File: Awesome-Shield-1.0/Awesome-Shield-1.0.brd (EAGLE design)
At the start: 51 x 55 mm, 21 parts, among them J1 PORT1, J2 PORT2, J3 PORT3, SW1 SPST_TACT-EVQQ2, SW2 DPDT, U1 LIGHTSENSORTEMT6000, X1 PASSER-07, X2 PASSER-07

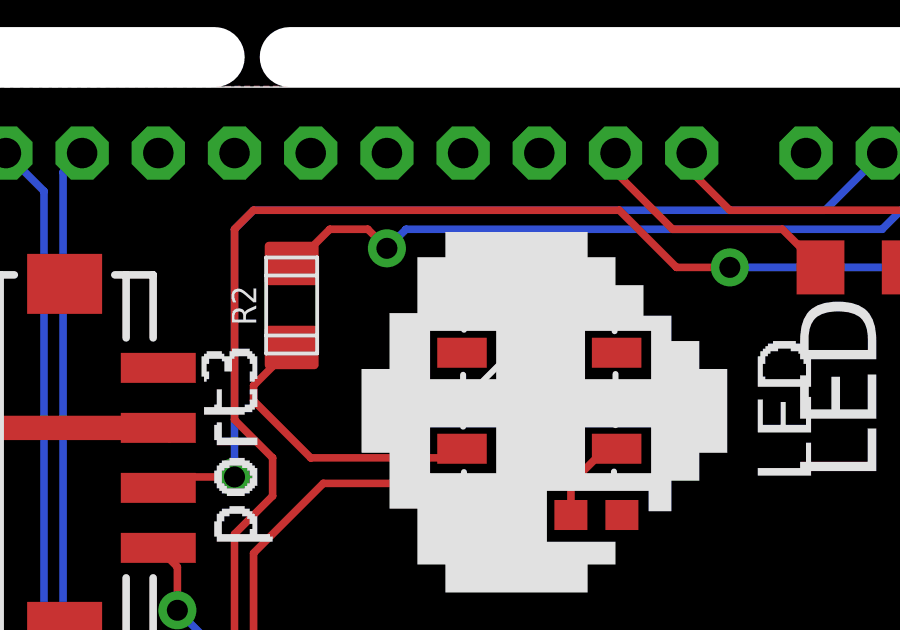
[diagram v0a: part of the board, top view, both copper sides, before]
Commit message: nudged resistor
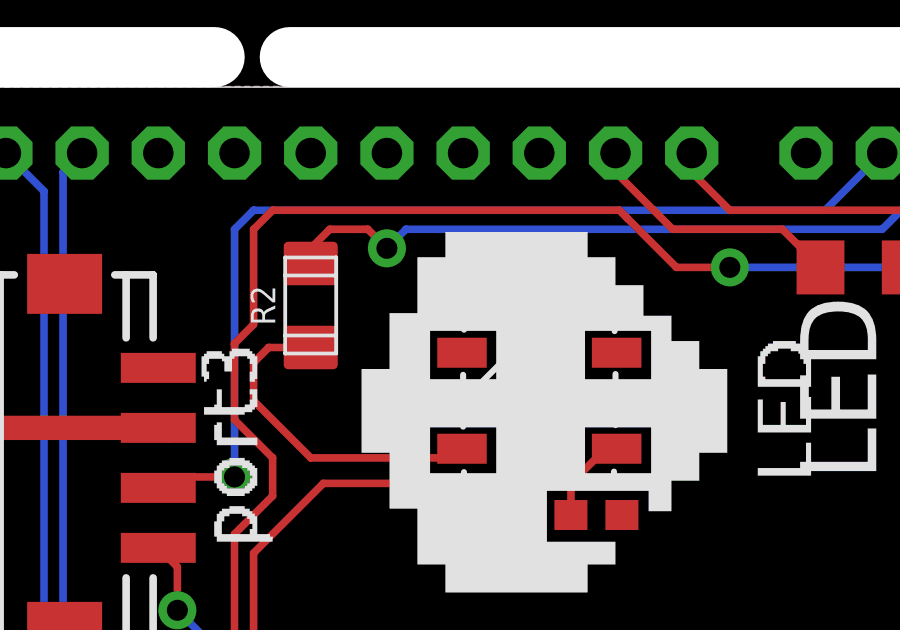
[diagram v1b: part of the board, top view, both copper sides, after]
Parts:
- moved R2 0.63 mm to (12.7, 45.7)
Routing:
- net N$3: track 10.2 -> 11.2 mm
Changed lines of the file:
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@@
 <element name="R1" library="rcl" package="R1206" value="TBD" x="31.115" y="46.99" smashed="yes" rot="R180"/>
 <element name="U$1" library="buzzer-loudity-bzel-t68-0808" package="SMT-68" value="LOUDITY-BZEL-T680808" x="38.735" y="43.18" smashed="yes" rot="R90"/>
-<element name="R2" library="we-rcl" package="C1206" value="330R" x="12.065" y="45.72"/>
+<element name="R2" library="we-rcl" package="C1206" value="330R" x="12.7" y="45.72"/>
 <element name="X1" library="we-symbol" package="PASSER_07MM" value="PASSER-07" x="1.27" y="48.26"/>
 <element name="X2" library="we-symbol" package="PASSER_07MM" value="PASSER-07" x="47.625" y="5.08"/>
@@
 <contactref element="R2" pad="1"/>
 <wire x1="13.335" y1="48.26" x2="12.195" y2="47.12" width="0.254" layer="1"/>
-<wire x1="12.195" y1="47.12" x2="12.065" y2="47.12" width="0.254" layer="1"/>
+<wire x1="12.195" y1="47.12" x2="12.7" y2="47.12" width="0.254" layer="1"/>
 <wire x1="13.335" y1="48.26" x2="14.605" y2="48.26" width="0.254" layer="1"/>
 <wire x1="14.605" y1="48.26" x2="15.24" y2="47.625" width="0.254" layer="1"/>
@@
 <wire x1="11.43" y1="39.37" x2="11.43" y2="40.64" width="0.254" layer="1"/>
 <wire x1="11.43" y1="40.64" x2="10.16" y2="41.91" width="0.254" layer="1"/>
-<wire x1="10.16" y1="41.91" x2="10.16" y2="48.26" width="0.254" layer="1"/>
-<wire x1="10.16" y1="48.26" x2="10.795" y2="48.895" width="0.254" layer="1"/>
-<wire x1="10.795" y1="48.895" x2="22.987" y2="48.895" width="0.254" layer="1"/>
-<wire x1="22.987" y1="48.895" x2="24.892" y2="46.99" width="0.254" layer="1"/>
+<wire x1="23.241" y1="48.641" x2="24.892" y2="46.99" width="0.254" layer="1"/>
 <wire x1="24.892" y1="46.99" x2="26.67" y2="46.99" width="0.254" layer="1"/>
 <via x="26.67" y="46.99" extent="1-16" drill="0.7" diameter="1.27"/>
 <wire x1="26.67" y1="46.99" x2="35.56" y2="46.99" width="0.254" layer="16"/>
 <wire x1="35.56" y1="46.99" x2="39.37" y2="50.8" width="0.254" layer="16"/>
+<wire x1="10.16" y1="41.91" x2="10.16" y2="44.45" width="0.254" layer="1"/>
+<wire x1="10.16" y1="44.45" x2="10.795" y2="45.085" width="0.254" layer="1"/>
+<wire x1="10.795" y1="45.085" x2="10.795" y2="48.26" width="0.254" layer="1"/>
+<wire x1="10.795" y1="48.26" x2="11.43" y2="48.895" width="0.254" layer="1"/>
+<wire x1="11.43" y1="48.895" x2="22.987" y2="48.895" width="0.254" layer="1"/>
+<wire x1="22.987" y1="48.895" x2="23.241" y2="48.641" width="0.254" layer="1"/>
 </signal>
 <signal name="A3">
@@
 <contactref element="R2" pad="2"/>
 <contactref element="D1" pad="4"/>
-<wire x1="12.065" y1="44.32" x2="10.795" y2="43.05" width="0.254" layer="1"/>
-<wire x1="10.795" y1="43.05" x2="10.795" y2="42.545" width="0.254" layer="1"/>
 <wire x1="10.795" y1="42.545" x2="12.7" y2="40.64" width="0.254" layer="1"/>
 <wire x1="12.7" y1="40.64" x2="17.438" y2="40.64" width="0.254" layer="1"/>
 <wire x1="17.438" y1="40.64" x2="17.743" y2="40.945" width="0.254" layer="1"/>
+<wire x1="12.7" y1="44.32" x2="11.3" y2="44.32" width="0.254" layer="1"/>
+<wire x1="11.3" y1="44.32" x2="10.795" y2="43.815" width="0.254" layer="1"/>
+<wire x1="10.795" y1="43.815" x2="10.795" y2="42.545" width="0.254" layer="1"/>
 </signal>
 </signals>
